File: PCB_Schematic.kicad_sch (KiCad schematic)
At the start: 59 parts, among them J1 USB_A, J2 Conn_02x05_Odd_Even, J3 Conn_02x03_Odd_Even, J4 Conn_02x03_Odd_Even, Q7 BSS138, SW1 SW_Push, U2 LM1117MP-ADJ, U3 TPS54331-Q1, U5 FT232RL, U6 STM32F091RCTx, X1 32.768kHz(12.5pF), X2 8MHz(20pF)

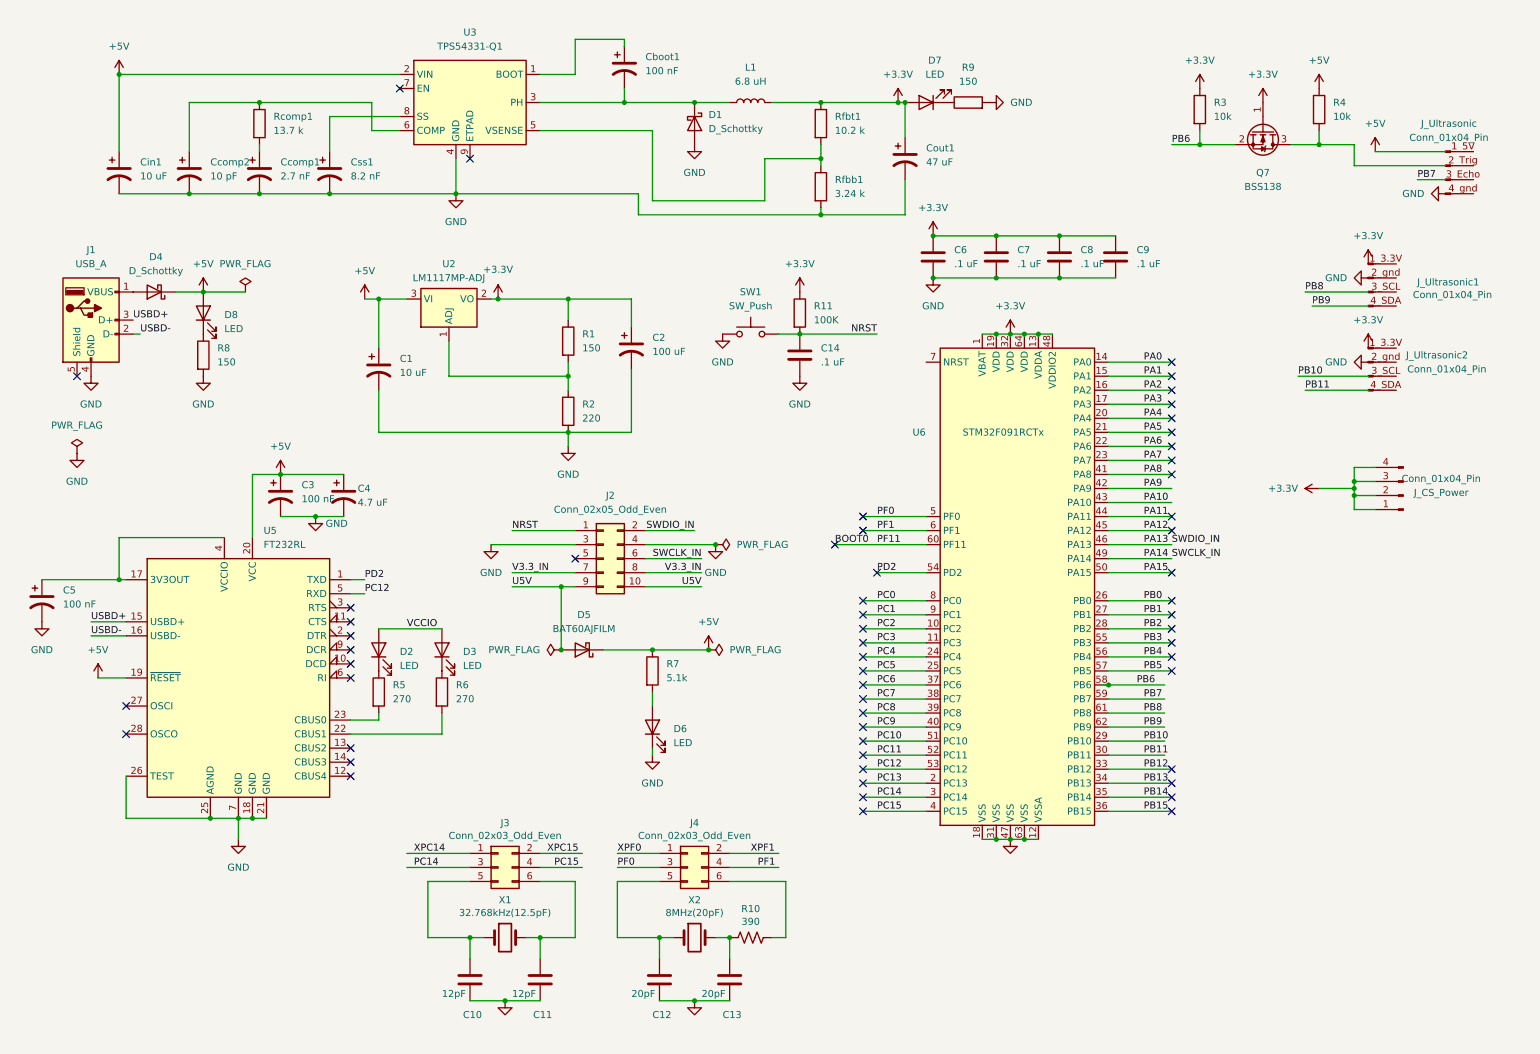
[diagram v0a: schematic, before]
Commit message: changes Sam
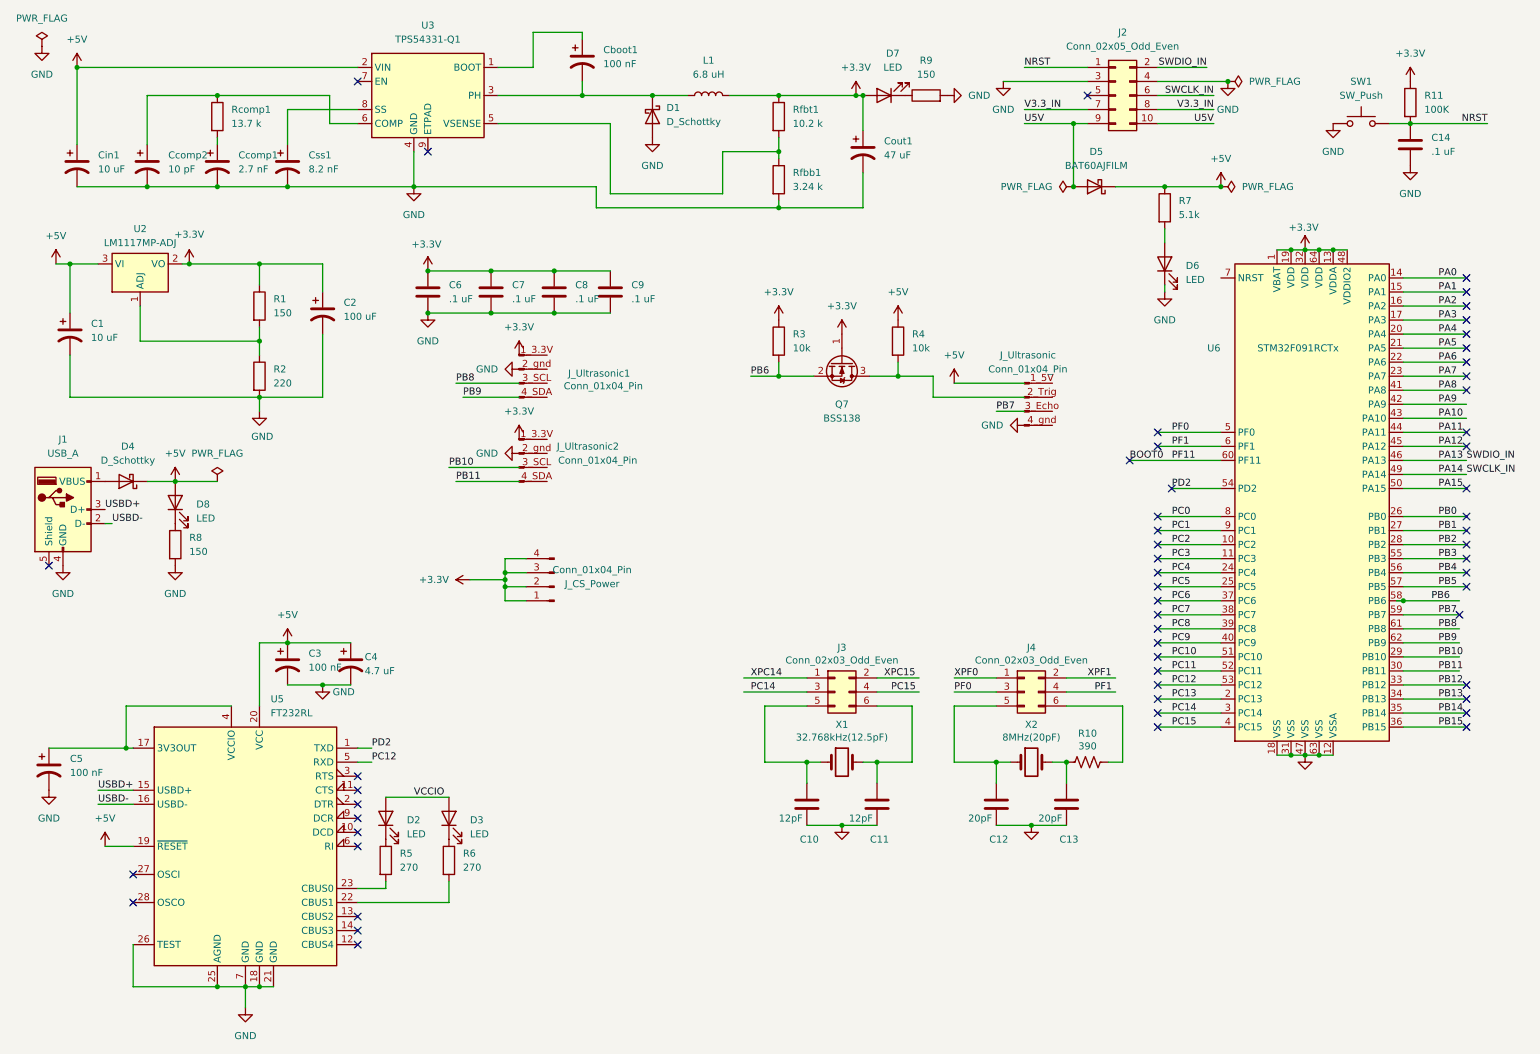
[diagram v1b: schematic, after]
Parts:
- C1, C14, C2, C3, C4, C5, C6, C7, C8, C9, Cboot1, Ccomp1, Ccomp2, Cin1, Css1: footprint (none) -> Capacitor_SMD:C_1206_3216Metric_Pad1.33x1.80mm_HandSolder
- R1, R11, R2, R3, R4, R5, R6, R7, R8, R9, Rcomp1, Rfbb1, Rfbt1: footprint (none) -> Resistor_SMD:R_1206_3216Metric_Pad1.30x1.75mm_HandSolder
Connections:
- no-connect marks 57 -> 58
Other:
- moved on the sheet: C1, C10, C11, C12, C13, C14, C2, C3, C4, C5, C6, C7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
